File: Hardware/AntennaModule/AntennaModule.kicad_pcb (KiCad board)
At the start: 4 copper layers, 80 x 80 mm, 53 parts, among them J1 Conn_01x10, SW1 ColdStart, U1 C0727J5003AHF-1, U2 C0727J5003AHF-1, U3 NJG1155UX2, U4 NT1192FAAE1S, U5 PD0922J5050S2HF, U6 NT1192FAAE1S, U7 NEO-D9C, U8 NEO-F9P, X1 TA1985A, X2 TE0133B

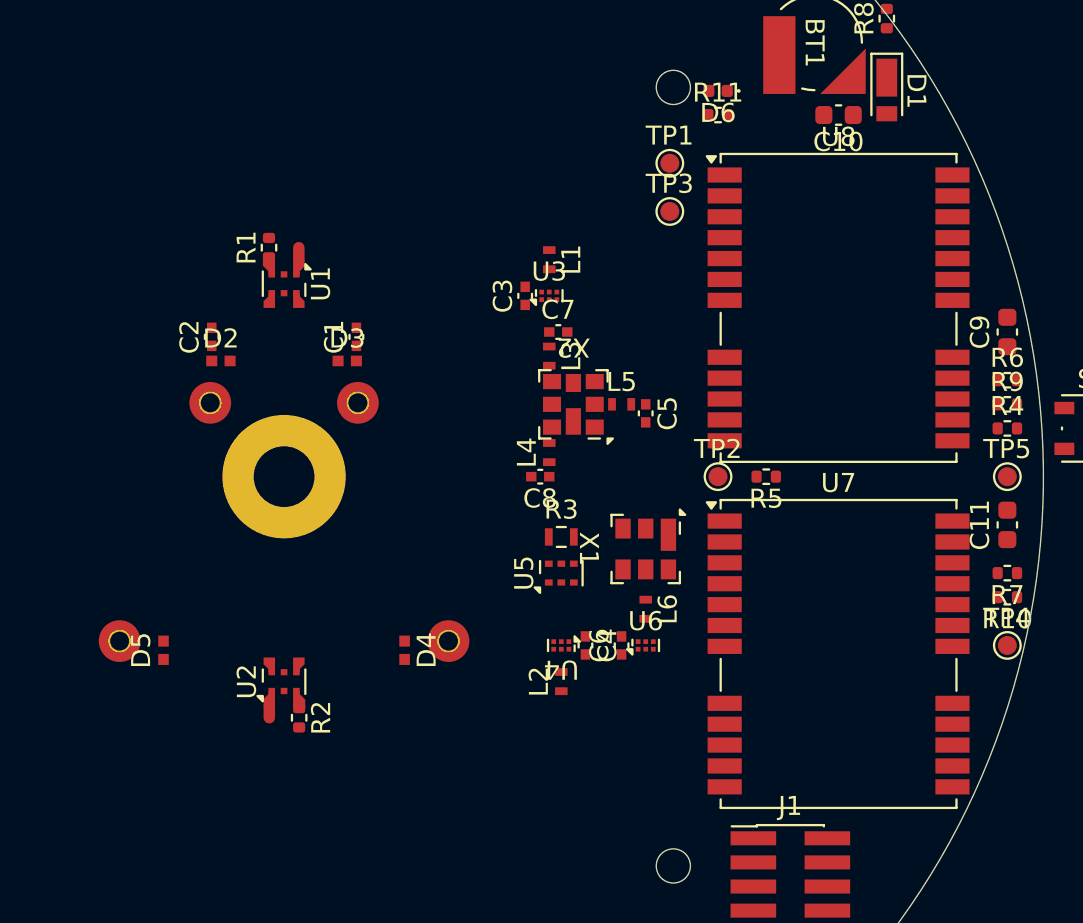
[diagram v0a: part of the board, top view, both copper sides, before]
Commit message: 配線中
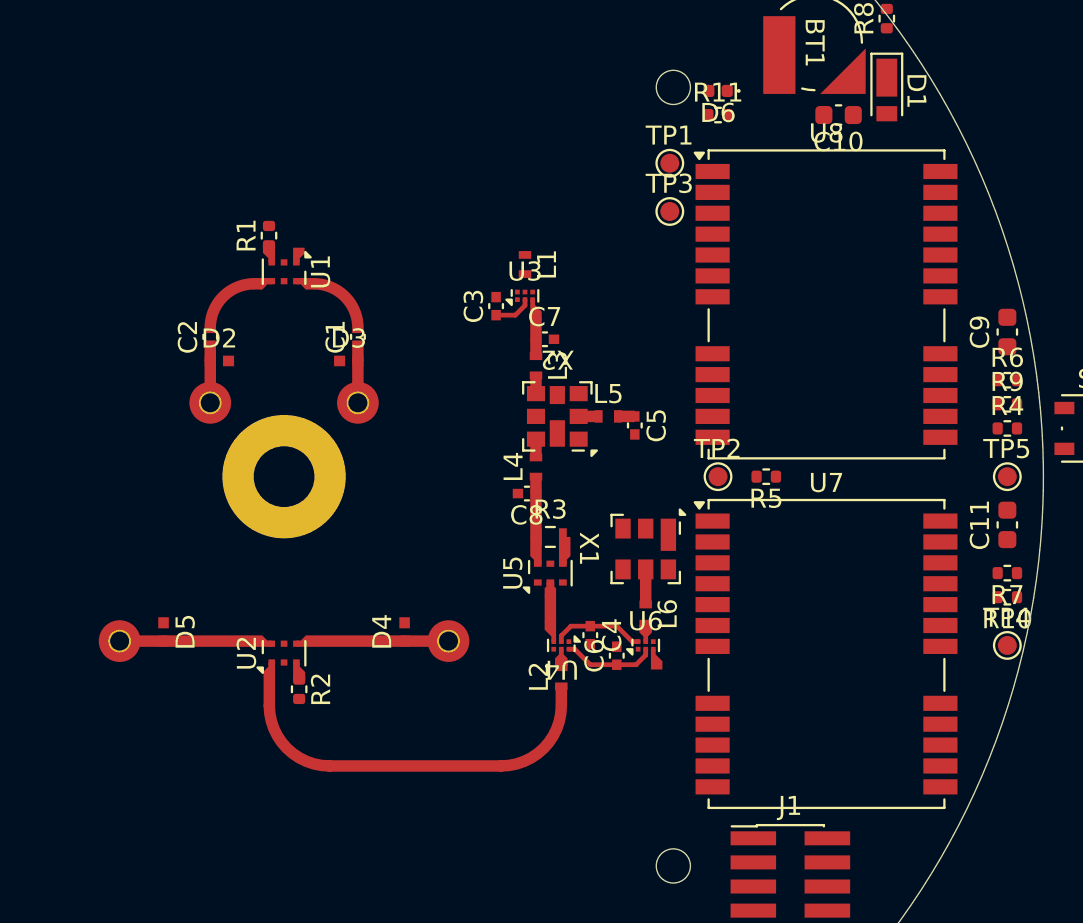
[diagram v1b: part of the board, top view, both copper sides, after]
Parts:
- moved C3 1.62 mm to (161.2, 91.0)
- moved R2 1.50 mm to (150.8, 111.2)
- moved U2 1.50 mm to (150.0, 109.3)
- moved L1 1.30 mm to (162.7, 88.8)
- moved U3 1.28 mm to (162.7, 90.5)
- moved C8 1.13 mm to (162.8, 100.9)
- moved X2 1.06 mm to (164.4, 96.8)
- moved L4 1.03 mm to (163.3, 99.5)
- moved D4 0.97 mm to (156.3, 108.2), turned to 90 degrees
- moved D5 0.97 mm to (143.7, 108.2), turned to -90 degrees
- moved L5 0.95 mm to (167.1, 96.8)
- moved L3 0.86 mm to (163.3, 94.2)
- moved C5 0.86 mm to (168.5, 97.3)
- moved C7 0.80 mm to (163.7, 92.8)
- moved U8 0.66 mm to (178.6, 90.9)
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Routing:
- net Net-(U2-Input): track 0.64 -> 20.3 mm
- net +3.3VA: track 0.00 -> 9.80 mm
- net Net-(AE1B-LB2): track 0.00 -> 2.31 mm
- net Net-(AE1B-LB1): track 0.00 -> 2.31 mm
- net Net-(U5-Output2): track 0.00 -> 2.29 mm
- net Net-(AE1A-HB2): track 0.00 -> 2.21 mm
- net Net-(AE1A-HB1): track 0.00 -> 2.21 mm
- net +3.3VP: track 0.00 -> 2.04 mm
- net Net-(U4-RFOUT): track 0.00 -> 1.27 mm
- net Net-(U3-RFOUT): track 0.00 -> 1.02 mm
- net Net-(U1-Input): track 0.63 -> 0.00 mm
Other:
- board text added: "上カプラは25milグリッドから0.0025mm下にずれてる"
